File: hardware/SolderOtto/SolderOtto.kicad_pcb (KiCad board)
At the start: 4 copper layers, 169.6 x 84 mm, 222 parts, among them J201 Conn_02x04_Counter_Clockwise, J301 TC-2050, J401 Conn_01x20, J501 Conn_01x08, J601 Conn_01x07, P301 USB_C_Plug_USB2.0, Q201 T2N7002AK, Q202 BC858B, Q203 BC847A, Q204 BC847A, Q801 Q_Dual_NMOS, Q802 Q_Dual_NMOS, Q803 Q_Dual_NMOS, Q804 DTD123EK, Q805 DTD123EK, Q806 DTD123EK, Q807 Q_Dual_NMOS, Q808 Q_Dual_NMOS, Q809 DTD123EK, Q810 DTD123EK, Q901 BC847A, Q902 BC858B, Q903 BC847A, SW301 SW_Push, U201 LM5012, U202 AP3211K, U203 AP3211K, U204 AP3211K, U205 LM27761, U206 MCP9701T-E/TT, U301 USBLC6-2SC6, U302 STM32G474QETx, U303 MX25R3235FM1xx0, U701 SN74LVC125A, U702 TS5A3159ADCK, U801 VOM1271, U802 VOM1271, U803 VOM1271, U804 VOM1271, U805 VOM1271, U901 OP07, U902 LM358, U903 74hc4053, U904 OP07, U905 OP07, Y301 32.768 kHz

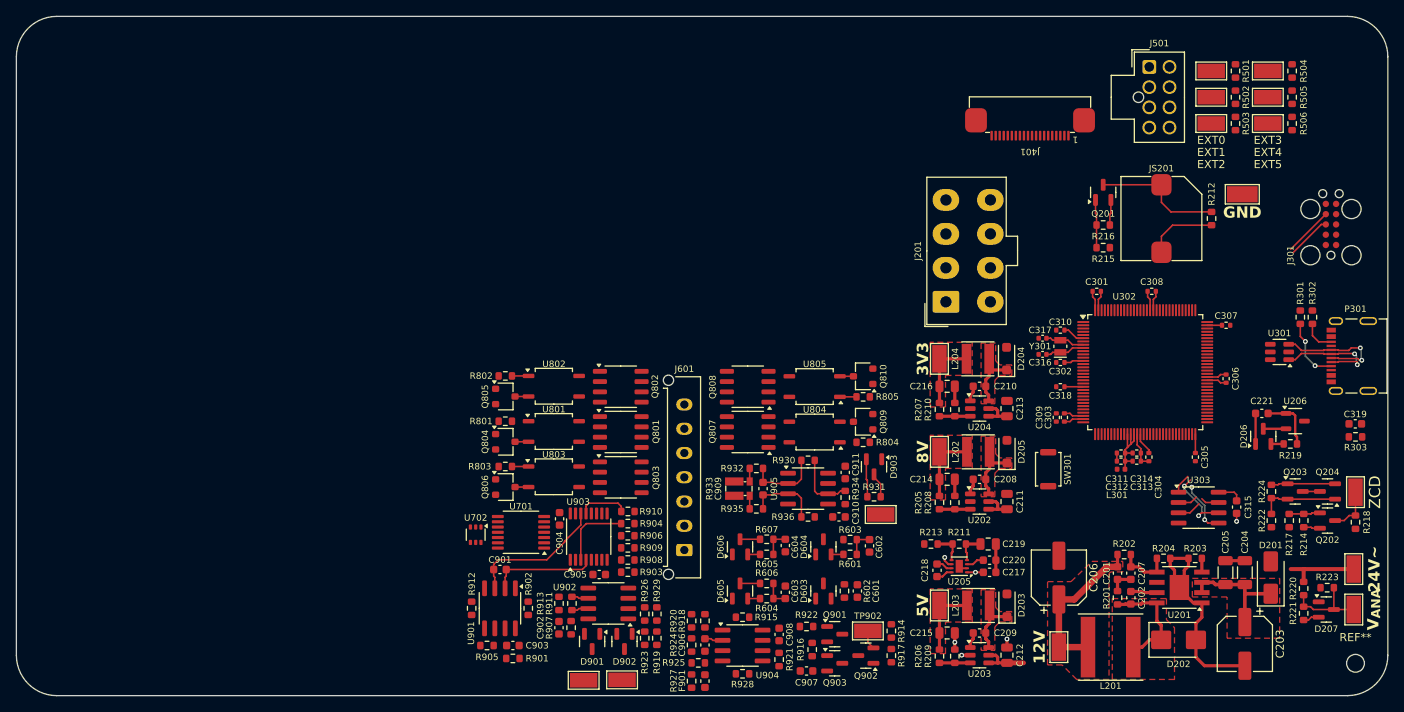
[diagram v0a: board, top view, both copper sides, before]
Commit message: save work
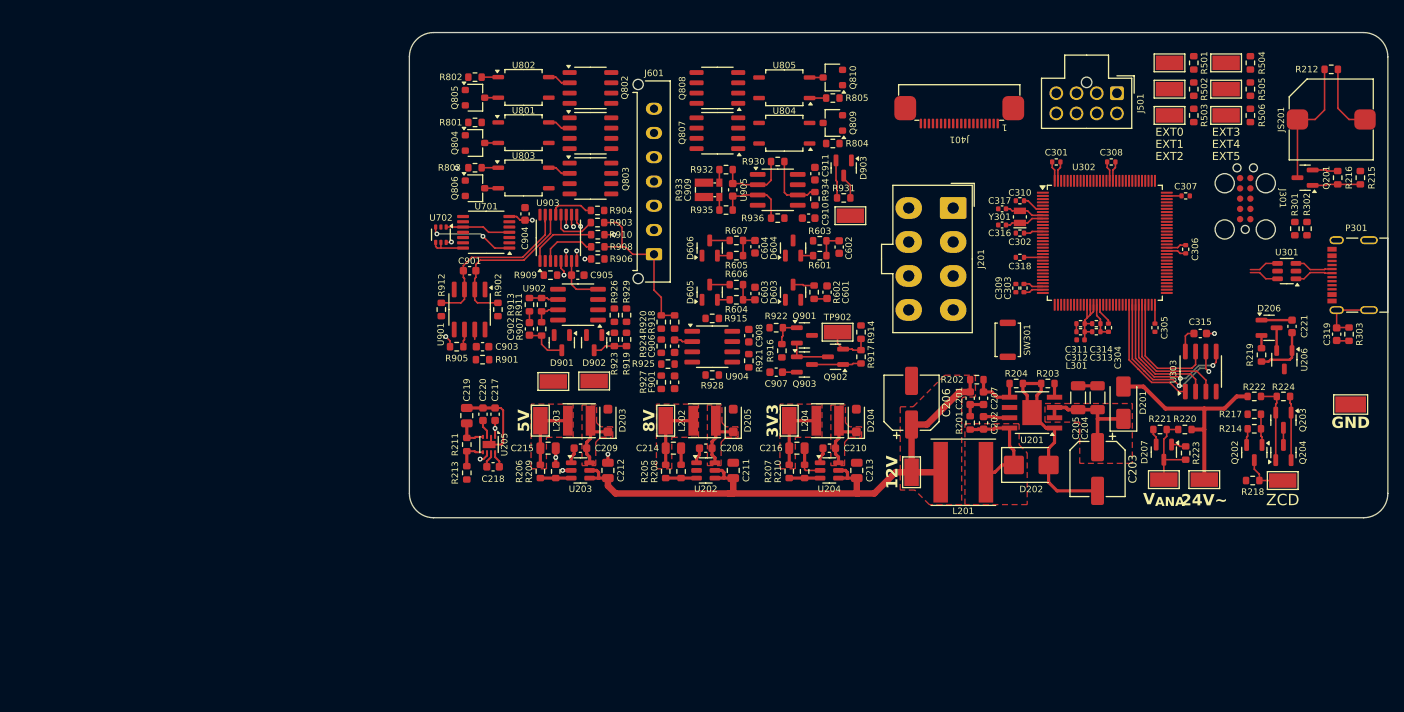
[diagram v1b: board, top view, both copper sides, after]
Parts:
- removed REF**: MountingHole_2.2mm_M2, MountingHole:MountingHole_2.2mm_M2
- moved C219 66.4 mm to (116.1, 97.4), turned to 90 degrees
- moved C220 65.2 mm to (118.1, 97.2), turned to 90 degrees
- moved C217 64.2 mm to (119.6, 97.2), turned to 90 degrees
- moved R211 62.1 mm to (116.1, 101.0), turned to -90 degrees
- moved U205 60.1 mm to (118.8, 101.0), turned to -90 degrees
- moved R213 58.1 mm to (116.1, 104.5), turned to -90 degrees
- moved C218 56.4 mm to (119.3, 103.7), turned to 180 degrees
- moved R206 54.4 mm to (125.2, 104.3)
- moved TP205 54.4 mm to (125.2, 98.0)
- moved C209 54.4 mm to (130.2, 101.4)
- moved C212 54.4 mm to (133.6, 104.2)
- moved C215 54.4 mm to (126.2, 101.4)
- moved D203 54.4 mm to (133.6, 98.0)
- moved L203 54.4 mm to (130.0, 98.0)
- moved R209 54.4 mm to (127.1, 104.3)
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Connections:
- C901 pad 1: Net-(U901--) -> /Channel0/channel_meas/IN-
- R902 pad 1: Net-(U901--) -> /Channel0/channel_meas/IN-
- R903 pad 2: Net-(U903-3Y0) -> Net-(U903-1Y0)
- R904 pad 2: Net-(U903-3Y1) -> Net-(U903-1Y1)
- R906 pad 1: /Channel0/LOAD -> /Channel0/_iron_sense
- R906 pad 2: Net-(U903-2Y0) -> Net-(U903-3Y0)
- R908 pad 2: Net-(U903-2Y1) -> Net-(U903-3Y1)
- R909 pad 2: Net-(U903-1Y0) -> Net-(U903-2Y0)
- R910 pad 1: /Channel0/_iron_sense -> /Channel0/LOAD
- R910 pad 2: Net-(U903-1Y1) -> Net-(U903-2Y1)
- U901 pad 2: Net-(U901--) -> /Channel0/channel_meas/IN-
- U903 pad 11: /Channel0/SEL1 -> /Channel0/SEL3
- U903 pad 14: Net-(U901-+) -> /Channel0/channel_meas/IN-
- U903 pad 15: /Channel0/channel_meas/select -> Net-(U901-+)
- U903 pad 4: Net-(U901--) -> /Channel0/channel_meas/select
- U903 pad 9: /Channel0/SEL3 -> /Channel0/SEL1
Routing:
- net +12V: track 34.5 -> 77.0 mm, vias 0 -> 1
- net GND: track 70.9 -> 94.8 mm, vias 4 -> 7
- net /Channel0/TC: track 0.00 -> 20.9 mm
- net /Channel0/channel_meas/IN-: track 0.00 -> 20.6 mm
- net 24V_{AC}: track 9.37 -> 27.5 mm
- net /mcu/QSPI_IO2: track 2.99 -> 16.9 mm
- net /mcu/QSPI_IO1: track 2.45 -> 16.2 mm
- net Net-(U901--): track 13.2 -> 0.00 mm
- net /mcu/QSPI_CLK: track 2.41 -> 15.4 mm
- net /mcu/QSPI_IO0: track 6.87 -> 19.8 mm
- net /mcu/QSPI_NCS: track 8.42 -> 21.2 mm
- net /mcu/QSPI_IO3: track 2.27 -> 15.0 mm
- net /Channel0/channel_power/COM_SW_LOW: track 0.00 -> 10.6 mm, vias 0 -> 2
- net /mcu/_D+: track 14.8 -> 4.80 mm, vias 2 -> 0
- net /mcu/_D-: track 13.6 -> 4.80 mm, vias 2 -> 0
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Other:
- board size 169.6 x 84 mm -> 121 x 60 mm
